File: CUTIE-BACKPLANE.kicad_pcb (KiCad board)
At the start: 4 copper layers, 57.5 x 86 mm, 22 parts, among them J1 ERF8-025-05.0-L-DV-L-K-TR, J2 ERF8-025-05.0-L-DV-L-K-TR, J3 ERF8-025-05.0-L-DV-L-K-TR, J4 ERF8-025-05.0-L-DV-L-K-TR, J7 USB3_A

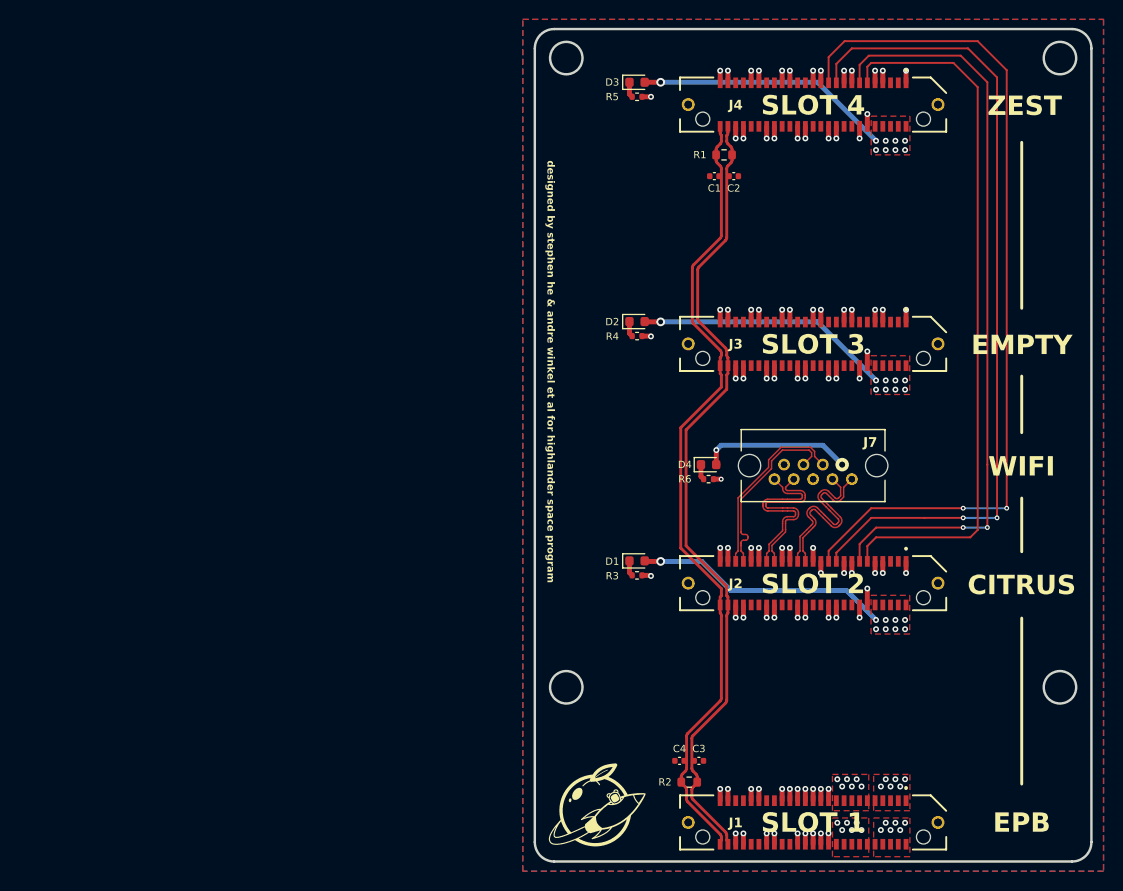
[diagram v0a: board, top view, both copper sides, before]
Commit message: added tps and new init layout
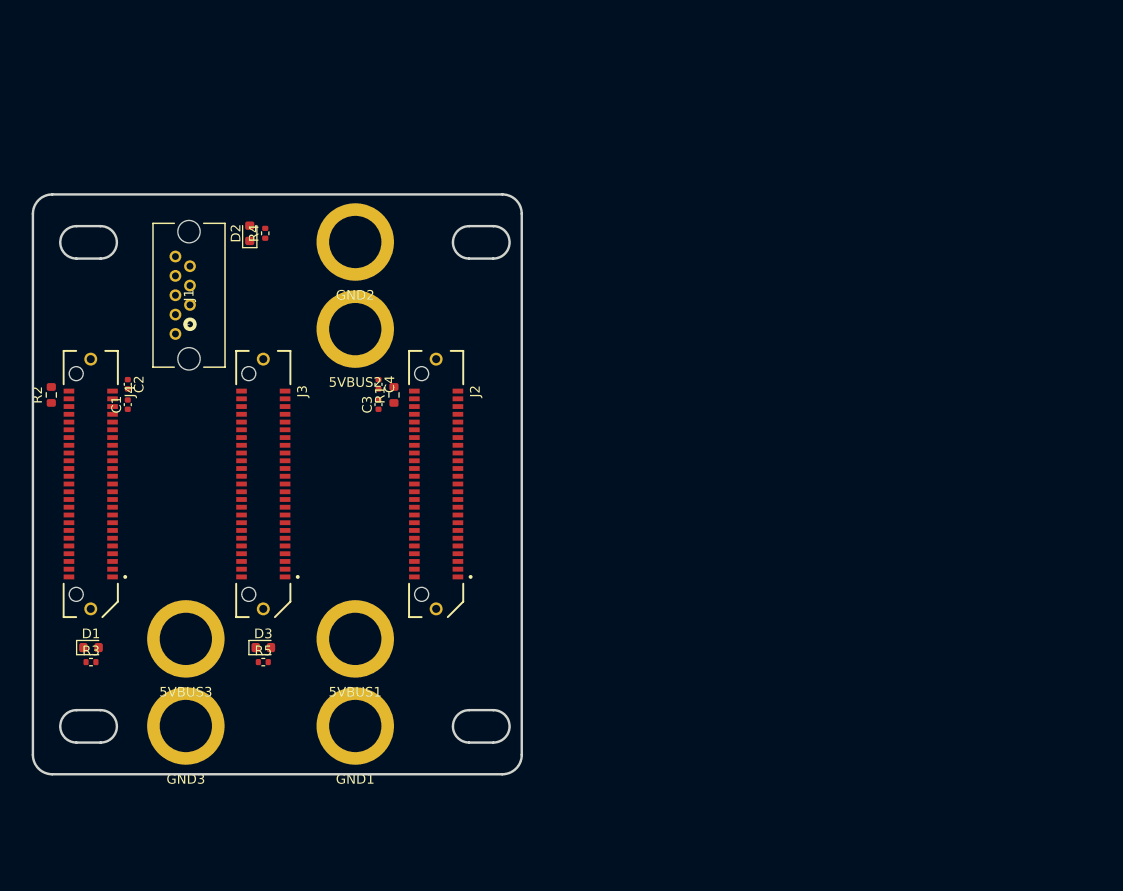
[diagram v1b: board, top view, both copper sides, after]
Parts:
- removed D4: LED Red, LED_SMD:LED_0603_1608Metric
- removed G*** (x3): LOGO, LOGO
- removed J7: USB3_A, library:CONN9_08-0003_MOL
- removed R6: 1k, Resistor_SMD:R_0402_1005Metric
- added 5VBUS1: TestPoint, library:KEYSTONE_575-4, F.Cu at (105.7, 112.0)
- added 5VBUS2: TestPoint, library:KEYSTONE_575-4, F.Cu at (105.7, 80.0)
- added 5VBUS3: TestPoint, library:KEYSTONE_575-4, F.Cu at (88.2, 112.0)
- added GND1: TestPoint, library:KEYSTONE_575-4, F.Cu at (105.7, 121.0)
- added GND2: TestPoint, library:KEYSTONE_575-4, F.Cu at (105.7, 71.0)
- added GND3: TestPoint, library:KEYSTONE_575-4, F.Cu at (88.2, 121.0)
- J1: value ERF8-025-05.0-L-DV-L-K-TR -> USB3_A; footprint library:SAMTEC_ERF8-025-05.0-L-DV-L-K-TR -> library:CONN9_08-0003_MOL
- R3, R4, R5: value 1k -> 330
- moved J4 84.3 mm to (78.4, 96.0), turned to -90 degrees
- moved J1 82.4 mm to (88.6, 79.5), turned to 90 degrees
- moved R2 77.1 mm to (74.3, 86.8), turned to 90 degrees
- moved D3 70.0 mm to (96.2, 112.9)
- moved R5 70.0 mm to (96.2, 114.4)
- moved C2 66.2 mm to (82.2, 85.7), turned to -90 degrees
- moved C1 65.0 mm to (82.2, 87.8), turned to 90 degrees
- moved J3 58.6 mm to (96.2, 96.0), turned to -90 degrees
- moved D1 57.1 mm to (78.4, 112.9)
- moved R3 57.1 mm to (78.4, 114.4)
- moved C4 49.8 mm to (108.1, 85.7), turned to -90 degrees
- moved C3 49.5 mm to (108.1, 87.8), turned to 90 degrees
- moved R1 42.2 mm to (109.7, 86.8), turned to 90 degrees
- moved D2 41.0 mm to (94.8, 70.1), turned to 90 degrees
- moved J2 40.3 mm to (114.1, 96.0), turned to -90 degrees
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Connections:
- C1 pad 2: /Slot 1/CAN0.N -> /CITRUS/CAN0.P
- C2 pad 2: /Slot 1/CAN0.P -> /CITRUS/CAN0.N
- C3 pad 2: /Slot 1/CAN0.P -> /CITRUS/CAN0.P
- C4 pad 2: /Slot 1/CAN0.N -> /CITRUS/CAN0.N
- D1 pad 2: /Slot 1/5V0_1 -> /LEMON/5VBUS3
- D2 pad 2: /Slot 1/5V0_2 -> /LEMON/5VBUS2
- D3 pad 2: /Slot 1/5V0_3 -> /CITRUS/5V0
- J2 pad 02: /Slot 1/5V0_1 -> GND
- J2 pad 03: unconnected-(J2-Pad03) -> GND
- J2 pad 04: /Slot 1/5V0_1 -> GND
- J2 pad 05: unconnected-(J2-Pad05) -> GND
- J2 pad 06: /Slot 1/5V0_1 -> GND
- J2 pad 08: /Slot 1/5V0_1 -> GND
- J2 pad 10: /Slot 1/5V0_1 -> GND
- J2 pad 11: /Slot 2/CMRF.CS0n -> GND
- J2 pad 13: /Slot 2/CMRF.SCLK -> GND
- J2 pad 15: GND -> /LEMON/5VBUS3
- J2 pad 16: unconnected-(J2-Pad16) -> GND
- J2 pad 17: GND -> /LEMON/5VBUS3
- J2 pad 18: unconnected-(J2-Pad18) -> GND
- J2 pad 19: /Slot 2/CMRF.MISO -> /LEMON/5VBUS3
- J2 pad 21: /Slot 2/CMRF.MOSI -> /LEMON/5VBUS3
- J2 pad 24: unconnected-(J2-Pad24) -> GND
- J2 pad 26: unconnected-(J2-Pad26) -> GND
- J2 pad 27: /Slot 2/USB3.TX_P -> /LEMON/5VBUS2
- J2 pad 29: /Slot 2/USB3.TX_N -> /LEMON/5VBUS2
- J2 pad 31: GND -> /LEMON/5VBUS2
- J2 pad 32: unconnected-(J2-Pad32) -> GND
- J2 pad 33: GND -> /LEMON/5VBUS2
- J2 pad 34: unconnected-(J2-Pad34) -> GND
- J2 pad 35: /Slot 2/USB3.RX_P -> GND
- J2 pad 37: /Slot 2/USB3.RX_N -> GND
- J2 pad 39: GND -> /CITRUS/5V0
- J2 pad 40: unconnected-(J2-Pad40) -> GND
- J2 pad 41: GND -> /CITRUS/5V0
- J2 pad 42: unconnected-(J2-Pad42) -> GND
- J2 pad 43: /Slot 2/USB3.D_P -> /CITRUS/5V0
- J2 pad 45: /Slot 2/USB3.D_N -> /CITRUS/5V0
- J2 pad 48: /Slot 1/CAN0.P -> /CITRUS/CAN0.P
- J2 pad 50: /Slot 1/CAN0.N -> /CITRUS/CAN0.N
- J3 pad 02: /Slot 1/5V0_2 -> /CITRUS/5V0
- J3 pad 03: unconnected-(J3-Pad03) -> GND
- J3 pad 04: /Slot 1/5V0_2 -> /CITRUS/5V0
- J3 pad 05: unconnected-(J3-Pad05) -> GND
- J3 pad 06: /Slot 1/5V0_2 -> /CITRUS/5V0
- J3 pad 08: /Slot 1/5V0_2 -> /CITRUS/5V0
- J3 pad 10: /Slot 1/5V0_2 -> /CITRUS/5V0
- J3 pad 11: unconnected-(J3-Pad11) -> /CITRUS/CMRF.CS0n
- J3 pad 13: unconnected-(J3-Pad13) -> /CITRUS/CMRF.SCLK
- J3 pad 16: unconnected-(J3-Pad16) -> GND
- J3 pad 18: unconnected-(J3-Pad18) -> GND
- J3 pad 19: unconnected-(J3-Pad19) -> /CITRUS/CMRF.MISO
- J3 pad 21: unconnected-(J3-Pad21) -> /CITRUS/CMRF.MOSI
- J3 pad 24: unconnected-(J3-Pad24) -> GND
- J3 pad 26: unconnected-(J3-Pad26) -> GND
- J3 pad 27: unconnected-(J3-Pad27) -> /CITRUS/USB3.TX_P
- J3 pad 29: unconnected-(J3-Pad29) -> /CITRUS/USB3.TX_N
- J3 pad 32: unconnected-(J3-Pad32) -> GND
- J3 pad 34: unconnected-(J3-Pad34) -> GND
- J3 pad 35: unconnected-(J3-Pad35) -> /CITRUS/USB3.RX_P
- J3 pad 37: unconnected-(J3-Pad37) -> /CITRUS/USB3.RX_N
- J3 pad 40: unconnected-(J3-Pad40) -> GND
- J3 pad 42: unconnected-(J3-Pad42) -> GND
- J3 pad 43: unconnected-(J3-Pad43) -> /CITRUS/USB3.D_P
- J3 pad 45: unconnected-(J3-Pad45) -> /CITRUS/USB3.D_N
- J3 pad 48: /Slot 1/CAN0.P -> /CITRUS/CAN0.P
- J3 pad 50: /Slot 1/CAN0.N -> /CITRUS/CAN0.N
- J4 pad 02: /Slot 1/5V0_3 -> /LEMON/5VBUS3
- J4 pad 03: unconnected-(J4-Pad03) -> GND
- J4 pad 04: /Slot 1/5V0_3 -> /LEMON/5VBUS3
- J4 pad 05: unconnected-(J4-Pad05) -> GND
- J4 pad 06: /Slot 1/5V0_3 -> /LEMON/5VBUS3
- J4 pad 08: /Slot 1/5V0_3 -> /LEMON/5VBUS3
- J4 pad 10: /Slot 1/5V0_3 -> /LEMON/5VBUS3
- J4 pad 11: /Slot 2/CMRF.CS0n -> /CITRUS/CMRF.CS0n
- J4 pad 13: /Slot 2/CMRF.SCLK -> /CITRUS/CMRF.SCLK
- J4 pad 16: unconnected-(J4-Pad16) -> GND
- J4 pad 18: unconnected-(J4-Pad18) -> GND
- J4 pad 19: /Slot 2/CMRF.MISO -> /CITRUS/CMRF.MISO
- J4 pad 21: /Slot 2/CMRF.MOSI -> /CITRUS/CMRF.MOSI
- J4 pad 24: unconnected-(J4-Pad24) -> GND
- J4 pad 26: unconnected-(J4-Pad26) -> GND
- J4 pad 27: unconnected-(J4-Pad27) -> GND
- J4 pad 29: unconnected-(J4-Pad29) -> GND
- J4 pad 32: unconnected-(J4-Pad32) -> GND
- J4 pad 34: unconnected-(J4-Pad34) -> GND
- J4 pad 35: unconnected-(J4-Pad35) -> GND
- J4 pad 37: unconnected-(J4-Pad37) -> GND
- J4 pad 40: unconnected-(J4-Pad40) -> GND
- J4 pad 42: unconnected-(J4-Pad42) -> GND
- J4 pad 43: unconnected-(J4-Pad43) -> GND
- J4 pad 45: unconnected-(J4-Pad45) -> GND
- J4 pad 48: /Slot 1/CAN0.P -> /CITRUS/CAN0.P
- J4 pad 50: /Slot 1/CAN0.N -> /CITRUS/CAN0.N
- R1 pad 1: /Slot 1/CAN0.P -> /CITRUS/CAN0.P
- R1 pad 2: /Slot 1/CAN0.N -> /CITRUS/CAN0.N
- R2 pad 1: /Slot 1/CAN0.P -> /CITRUS/CAN0.P
- R2 pad 2: /Slot 1/CAN0.N -> /CITRUS/CAN0.N
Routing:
- net GND: track 116.2 -> 0.00 mm, vias 93 -> 0
- net /Slot 2/CMRF.MOSI: track 89.5 -> 0.00 mm, vias 2 -> 0
- net /Slot 2/CMRF.MISO: track 84.9 -> 0.00 mm, vias 2 -> 0
- net /Slot 1/CAN0.P: track 84.0 -> 0.00 mm
- net /Slot 1/CAN0.N: track 84.0 -> 0.00 mm
- net /Slot 2/CMRF.SCLK: track 78.3 -> 0.00 mm, vias 2 -> 0
- net /Slot 2/CMRF.CS0n: track 73.7 -> 0.00 mm
- net /Slot 1/5V0_1: track 26.4 -> 0.00 mm, vias 15 -> 0
- net /Slot 1/5V0_2: track 26.4 -> 0.00 mm, vias 15 -> 0
- net /Slot 1/5V0_3: track 26.4 -> 0.00 mm, vias 15 -> 0
- net /Slot 2/USB3.D_N: track 19.1 -> 0.00 mm
- net /Slot 2/USB3.D_P: track 19.1 -> 0.00 mm
- net /Slot 2/USB3.RX_P: track 19.0 -> 0.00 mm
- net /Slot 2/USB3.RX_N: track 19.0 -> 0.00 mm
- net /Slot 2/USB3.TX_P: track 19.0 -> 0.00 mm
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- removed copper zone on F.Cu, net /Slot 1/5V0_1
- removed copper zone on In2.Cu, net /Slot 1/5V0_1
- removed copper zone on F.Cu, net /Slot 1/5V0_2
- removed copper zone on In2.Cu, net /Slot 1/5V0_2
- removed copper zone on F.Cu, net /Slot 1/5V0_3
- removed copper zone on In2.Cu, net /Slot 1/5V0_3
- removed copper zone on F.Cu, net /Slot 1/5V0_USB
- removed copper zone on In2.Cu, net /Slot 1/5V0_USB
- removed copper zone on B.Cu, net GND
- removed copper zone on F.Cu, net GND
- removed copper zone on In1.Cu, net GND
- removed copper zone on In2.Cu, net GND
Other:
- board size 57.5 x 86 mm -> 50.5 x 59.9 mm
- board text removed: "CITRUS"
- board text removed: "EMPTY"
- board text removed: "EPB"
- board text removed: "SLOT 1"
- board text removed: "SLOT 2"
- board text removed: "SLOT 3"
- board text removed: "SLOT 4"
- board text removed: "WIFI"
- board text removed: "ZEST"
- board text removed: "designed by stephen he & andre winkel et al for highlander space program"

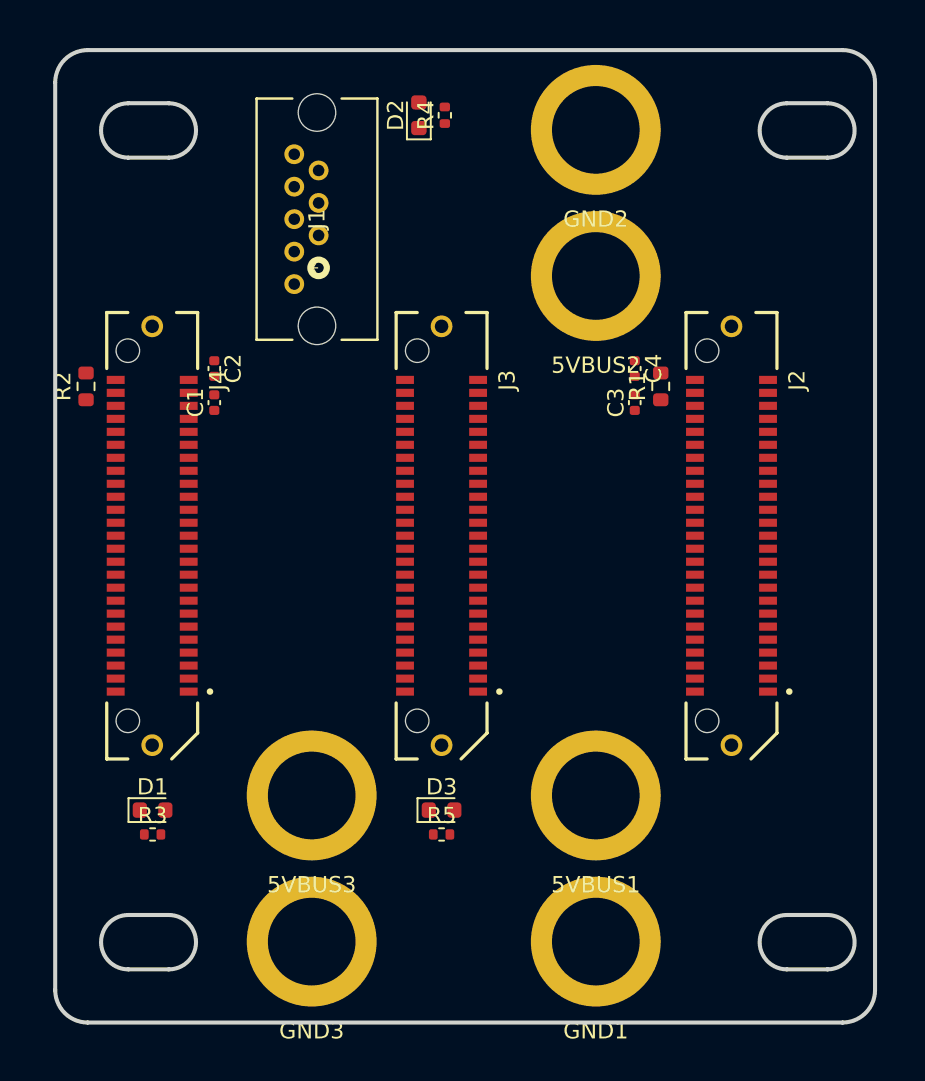
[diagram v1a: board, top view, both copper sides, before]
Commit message: layout complete pending review
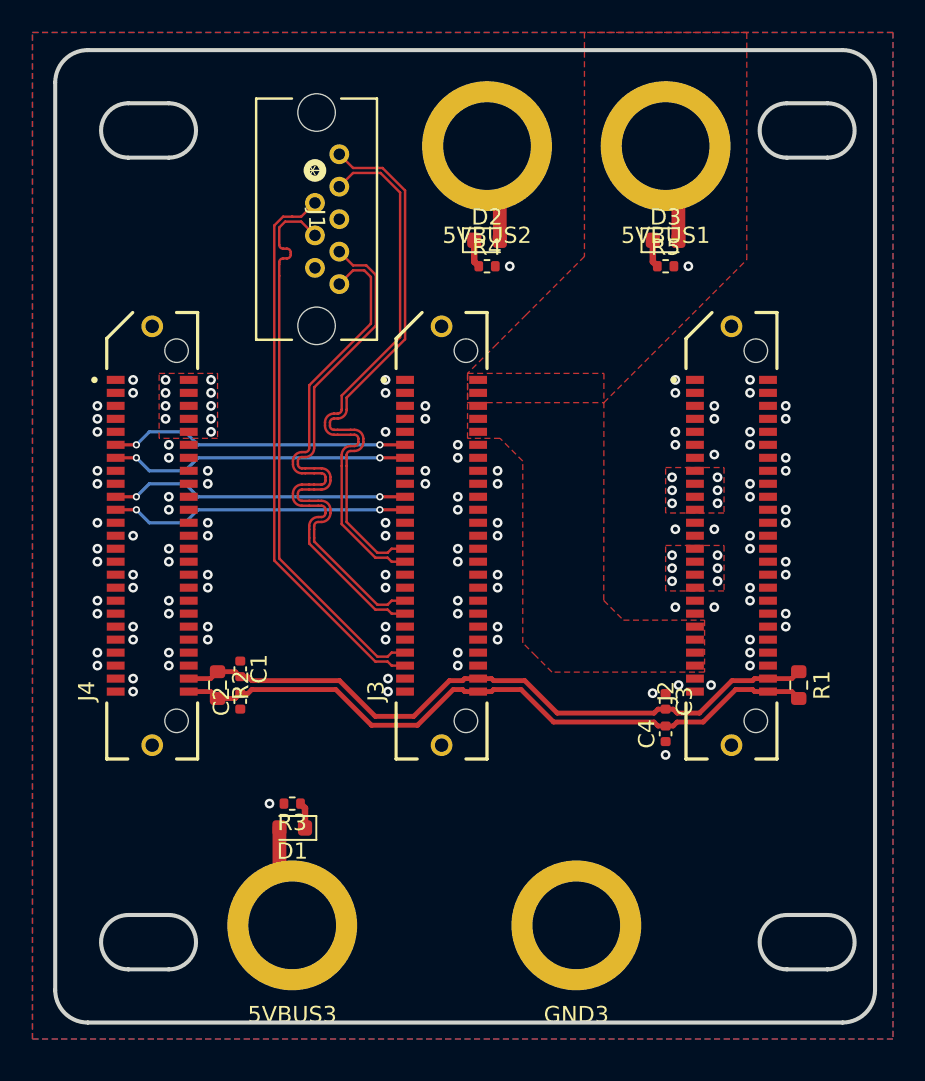
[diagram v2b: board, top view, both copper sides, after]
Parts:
- removed GND1, GND2: TestPoint, library:KEYSTONE_575-4
- moved 5VBUS1 40.2 mm to (110.0, 72.0)
- moved D3 37.7 mm to (110.0, 77.8)
- moved R5 37.6 mm to (110.0, 79.4)
- moved C4 22.6 mm to (110.0, 108.2), turned to 90 degrees
- moved C2 20.6 mm to (83.8, 106.2), turned to 90 degrees
- moved R1 20.3 mm to (118.2, 105.2), turned to -90 degrees
- moved R2 20.1 mm to (82.4, 105.2), turned to -90 degrees
- moved C3 18.5 mm to (110.0, 106.2), turned to -90 degrees
- moved C1 16.5 mm to (83.8, 104.2), turned to -90 degrees
- moved GND3 16.3 mm to (104.5, 120.0)
- moved 5VBUS2 10.4 mm to (99.0, 72.0)
- moved R4 9.66 mm to (99.0, 79.4), turned to 0 degrees
- moved R3 8.81 mm to (87.0, 112.5), turned to 180 degrees
- moved D2 8.77 mm to (99.0, 77.8), turned to 0 degrees
- moved D1 8.67 mm to (87.0, 114.0), turned to 180 degrees
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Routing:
- net /CITRUS/CAN0.N: track 0.00 -> 42.0 mm
- net /CITRUS/CAN0.P: track 0.00 -> 42.0 mm
- net /CITRUS/USB3.D_N: track 0.00 -> 34.5 mm
- net /CITRUS/USB3.D_P: track 0.00 -> 34.4 mm
- net /CITRUS/USB3.TX_P: track 0.00 -> 34.4 mm
- net /CITRUS/USB3.TX_N: track 0.00 -> 34.4 mm
- net /CITRUS/USB3.RX_P: track 0.00 -> 34.3 mm
- net /CITRUS/USB3.RX_N: track 0.00 -> 34.3 mm
- net /CITRUS/CMRF.CS0n: track 0.00 -> 18.5 mm, vias 0 -> 2
- net /CITRUS/CMRF.SCLK: track 0.00 -> 18.5 mm, vias 0 -> 2
- net /CITRUS/CMRF.MOSI: track 0.00 -> 18.5 mm, vias 0 -> 2
- net /CITRUS/CMRF.MISO: track 0.00 -> 18.5 mm, vias 0 -> 2
- net /LEMON/5VBUS3: track 0.00 -> 6.33 mm, vias 0 -> 15
- net /LEMON/5VBUS2: track 0.00 -> 6.13 mm, vias 0 -> 6
- net /CITRUS/5V0: track 0.00 -> 6.13 mm
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- added copper zone on F.Cu, net /CITRUS/5V0
- added copper zone on F.Cu, net /LEMON/5VBUS2
- added copper zone on In2.Cu, net /LEMON/5VBUS2
- added copper zone on F.Cu, net /LEMON/5VBUS3
- added copper zone on In2.Cu, net /LEMON/5VBUS3
- added copper zone on B.Cu, net GND
- added copper zone on F.Cu, net GND
- added copper zone on In1.Cu, net GND
- added copper zone on In2.Cu, net GND
